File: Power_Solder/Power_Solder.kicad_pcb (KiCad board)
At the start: 2 copper layers, 91.4 x 54.1 mm, 114 parts, among them IC1 MP1584EN, J1 HOTAIR HEAT, J2 HOTAIR SENSOR, J3 SOLDER HEAT, J4 SOLDER SENSOR, J5 220V IN, J6 24V IN, K1 FINDER-40.52, Q1 S8050, Q10 IRFR3708, Q2 S8050, Q3 S8050, Q4 S8550, Q5 IRFR3708, Q6 S8050, Q7 S8050, Q8 S8050, Q9 S8550, U1 LM358, U2 L7812, U3 Front Panel, U4 ACS712-05A, U5 ACS712-05A, U6 MOC3063M, U7 LTV-817S

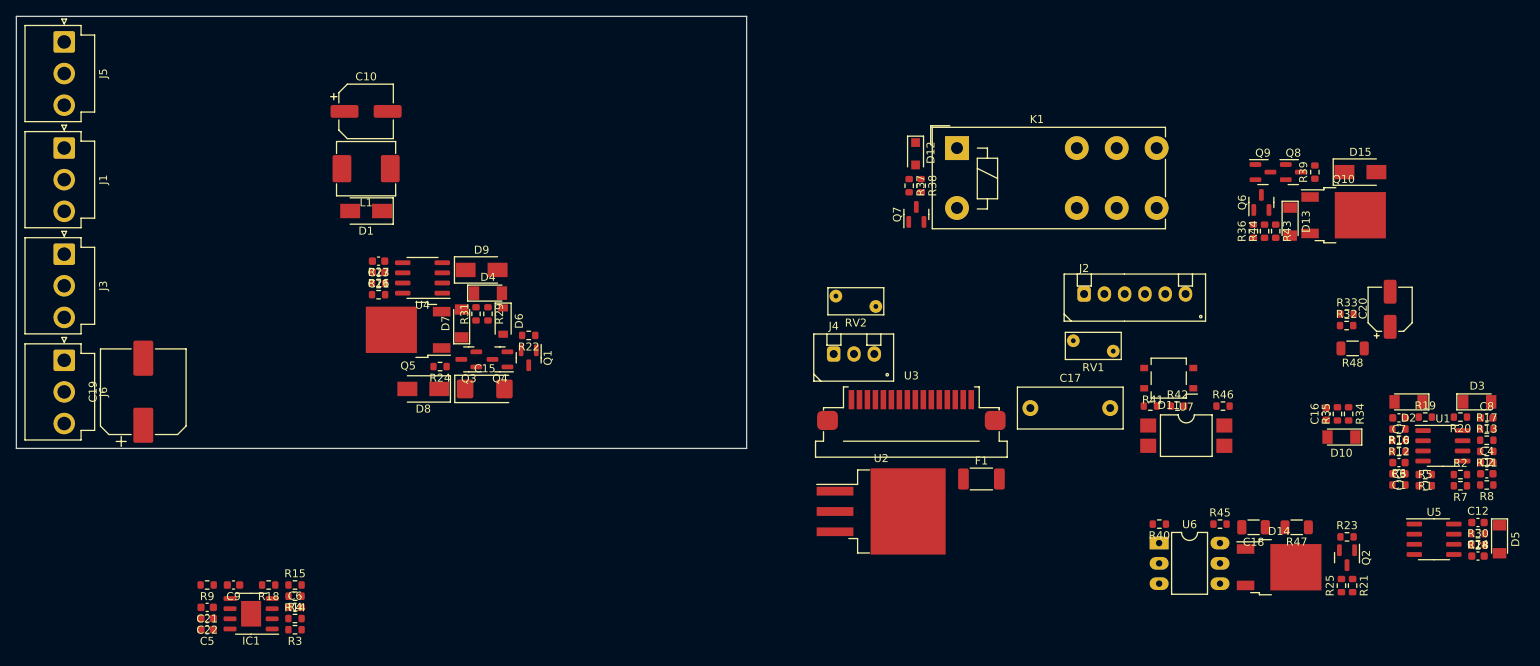
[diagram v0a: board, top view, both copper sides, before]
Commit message: Add files via upload
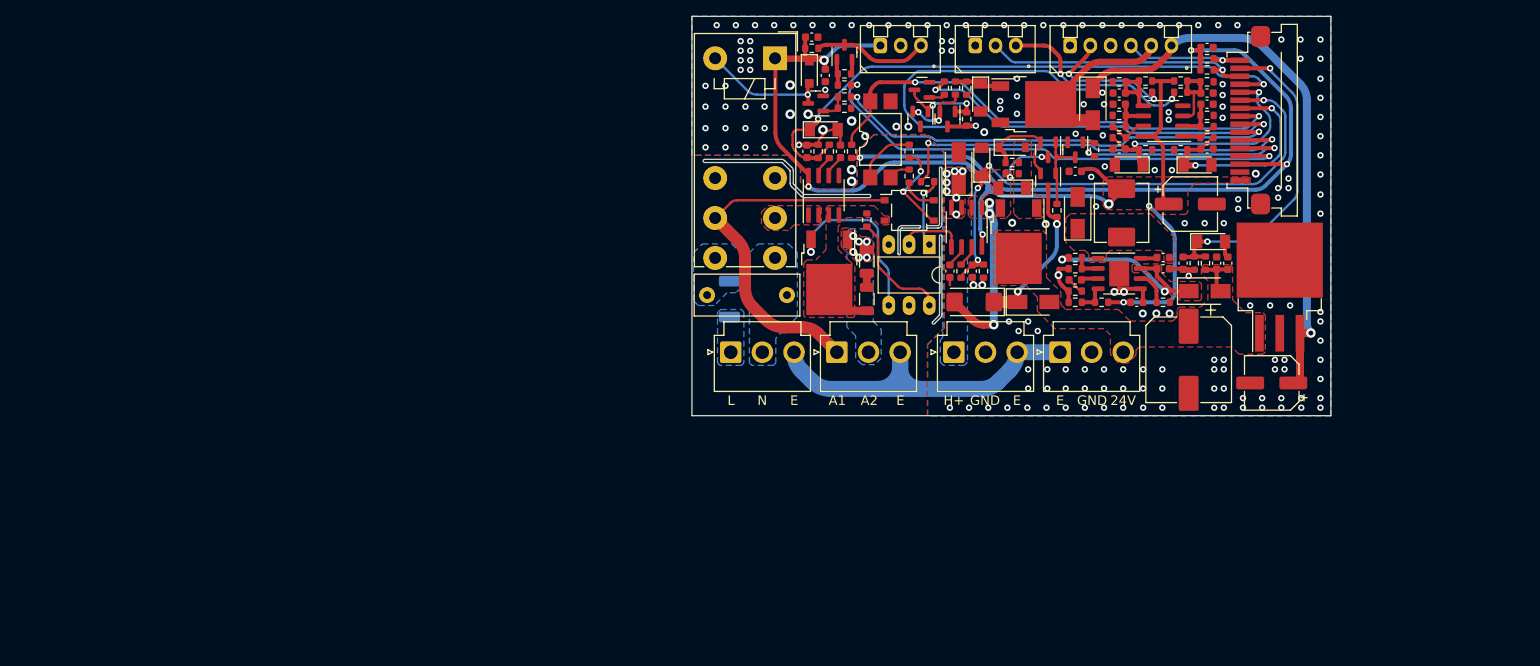
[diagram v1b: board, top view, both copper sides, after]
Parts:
- removed R48: 680k/1W, Resistor_SMD:R_1206_3216Metric
- removed RV1, RV2: VDR, Varistor:RV_Disc_D7mm_W3.4mm_P5mm
- added  : LOGO, Image:MVA_Bmpx20, B.Cu at (178.2, 102.3)
- added C23: 220uF, Capacitor_SMD:CP_Elec_6.3x7.7, F.Cu at (178.9, 119.3)
- added C24: 100nF, Capacitor_SMD:C_0603_1608Metric, F.Cu at (123.0, 80.8)
- added C25: 100nF, Capacitor_SMD:C_0603_1608Metric, F.Cu at (154.3, 92.8)
- added C26: 100nF, Capacitor_SMD:C_0603_1608Metric, F.Cu at (121.3, 76.0)
- added C27: 100nF, Capacitor_SMD:C_0603_1608Metric, F.Cu at (170.8, 77.3)
- added D16: SS34, Diode_SMD:D_SMA, F.Cu at (170.5, 107.8)
- added J7: SOLDER SENSOR, XH_2.54mm_Conn:XH_3P_2.54mm_Vertical, F.Cu at (129.9, 77.0)
- C20: value 47uF -> 1uF; footprint Capacitor_SMD:CP_Elec_5x5.4 -> Capacitor_SMD:C_0603_1608Metric
- F1: moved to B.Cu
- moved C22 135.3 mm to (173.4, 104.3), turned to 90 degrees
- moved C21 133.5 mm to (172.0, 104.3), turned to 90 degrees
- moved C19 131.0 mm to (168.5, 116.4), turned to -90 degrees
- moved C5 128.5 mm to (165.3, 103.6), turned to 0 degrees
- moved R9 124.8 mm to (165.3, 109.2), turned to 0 degrees
- moved J6 124.7 mm to (152.4, 115.5), turned to 0 degrees
- moved C9 118.5 mm to (162.0, 109.2), turned to 0 degrees
- moved IC1 116.7 mm to (159.8, 105.6), turned to 0 degrees
- moved J3 112.1 mm to (139.1, 115.5), turned to 0 degrees
- moved R18 110.1 mm to (157.6, 109.2), turned to 0 degrees
- moved R3 108.2 mm to (154.3, 103.6), turned to 0 degrees
- moved R4 107.1 mm to (154.3, 105.0), turned to 180 degrees
- moved C6 106.0 mm to (154.3, 106.4), turned to 180 degrees
- moved R14 104.9 mm to (154.3, 107.8)
- moved R15 103.9 mm to (154.3, 109.2), turned to 180 degrees
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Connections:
- C20 pad 1: +3.3V -> Net-(C20-Pad1)
- IC1 pad 7: +24V -> Net-(C20-Pad1)
- J1 pad 1: Earth_Protective -> AC2
- J1 pad 2: AC2 -> HOTAIR HEAT
- J1 pad 3: HOTAIR HEAT -> Earth_Protective
- J3 pad 1: Earth_Protective -> SOLDER HEAT
- J3 pad 3: SOLDER HEAT -> Earth_Protective
- J4 pad 2: VIBRA SENSOR -> SOLDER VIBRA
- J5 pad 1: Earth_Protective -> AC_L
- J5 pad 3: AC_L -> Earth_Protective
- K1 pad 11: Net-(C17-Pad1) -> AC1i
- K1 pad 14: AC2 -> AC_N
- K1 pad 21: AC_N -> AC2
- K1 pad 24: AC1i -> Net-(C17-Pad1)
- R3 pad 1: +24V -> Net-(C20-Pad1)
- U5 pad 1: AC1 -> AC1i
- U5 pad 2: AC1 -> AC1i
- U5 pad 3: AC1i -> AC1
- U5 pad 4: AC1i -> AC1
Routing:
- net +5V: track 0.00 -> 143.6 mm, vias 0 -> 6
- net +12V: track 0.00 -> 114.8 mm, vias 0 -> 3
- net +3.3V: track 0.00 -> 92.2 mm, vias 0 -> 3
- net HOTAIR CURRENT: track 0.00 -> 74.2 mm, vias 0 -> 2
- net SOLDER CURRENT: track 0.00 -> 67.7 mm, vias 0 -> 4
- net SPEAKER SW: track 0.00 -> 62.4 mm, vias 0 -> 2
- net ZERO CROSSING: track 0.00 -> 61.9 mm, vias 0 -> 2
- net POWER ENABLE: track 0.00 -> 56.6 mm, vias 0 -> 2
- net Earth_Protective: track 0.00 -> 54.8 mm
- net HOTAIR PWM: track 0.00 -> 53.0 mm, vias 0 -> 2
- net FAN PWM: track 0.00 -> 48.0 mm, vias 0 -> 2
- net AC2: track 0.00 -> 47.5 mm
- net VOLTAGE: track 0.00 -> 40.7 mm, vias 0 -> 2
- net GND: track 0.00 -> 40.1 mm, vias 0 -> 183
- net SOLDER VIBRA: track 0.00 -> 33.5 mm, vias 0 -> 1
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- added copper zone on F.Cu, net +24V
- added copper zone on F.Cu, net +5V
- added copper zone on F.Cu, net AC1
- added copper zone on F.Cu, net AC1i
- added copper zone on B.Cu, net AC_L
- added copper zone on B.Cu, net AC_N
- added copper zone on B.Cu, net GND
- added copper zone on F.Cu, net GND
- added copper zone on B.Cu, net HOTAIR HEAT
- added copper zone on F.Cu, net HOTAIR HEAT
- added copper zone on F.Cu, net Net-(C15-Pad2)
- added copper zone on B.Cu, net Net-(C17-Pad1)
- added copper zone on F.Cu, net Net-(C20-Pad1)
- added copper zone on F.Cu, net Net-(C5-Pad2)
- added copper zone on F.Cu, net Net-(D6-Pad2)
- added copper zone on B.Cu, net SOLDER HEAT
- added copper zone on F.Cu, net SOLDER HEAT
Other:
- board size 91.4 x 54.1 mm -> 80 x 50 mm
- board text added: "220VAC"
- board text added: "24V"
- board text added: "24VDC"
- board text added: "A1"
- board text added: "A2"
- board text added: "E"
- board text added: "FRONT PANEL"
- board text added: "GND"
- board text added: "H+"
- board text added: "HOTAIR"
- board text added: "L"
- board text added: "N"
- board text added: "SOLDER"
- board text added: "SPK"
